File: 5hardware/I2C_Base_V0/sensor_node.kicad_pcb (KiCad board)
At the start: 2 copper layers, 99.5 x 99.5 mm, 264 parts, among them J2 PJ-320D-A, J3 Conn_02x06_Top_Bottom, J4 Conn_01x19_Socket, J5 Conn_01x19_Socket, J6 Conn_01x06_Socket, J7 Conn_01x04_Pin, J8 Conn_01x04_Pin, P1 S3B-PH-SM4-TB, P2 S4B-PH-SM4-TB, P3 S3B-PH-SM4-TB, Q2 Si2371EDS, Q3 Si2371EDS, SW2 SW_Push, SW3 SW_Push, U10 ESP-12F, U12 APDS-9960, U14 DS3231M, U3 CR2450, U4 CH32V003F4P6, U5 SHT31-DIS, U6 DS1307Z+, U7 XC6206PxxxMR, U8 TPL5110, U9 BH1750FVI-TR, Y1 Crystal, Y2 Crystal

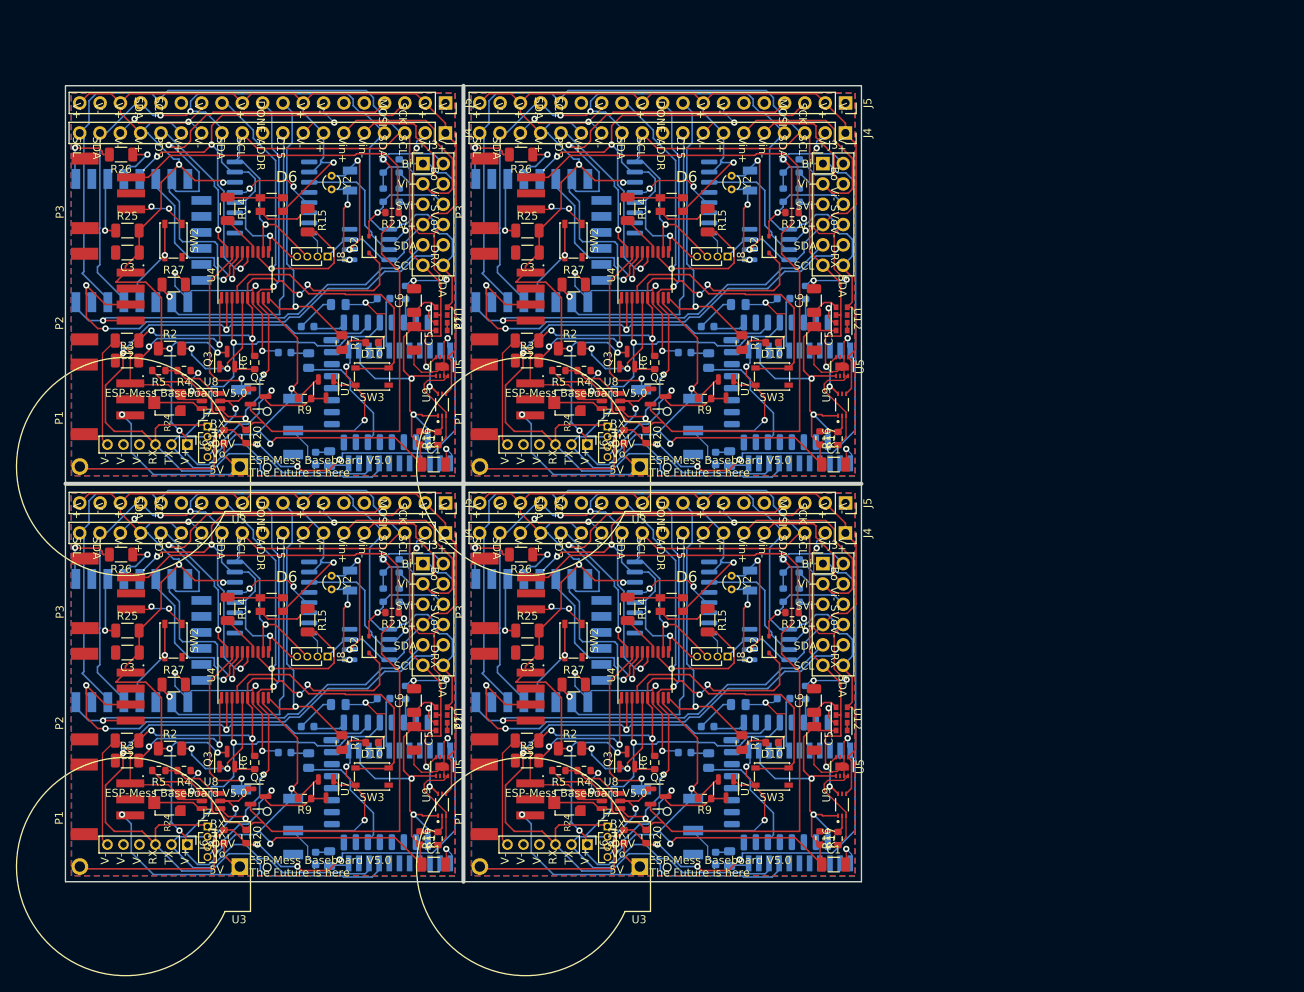
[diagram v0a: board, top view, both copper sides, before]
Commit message: update PCB.
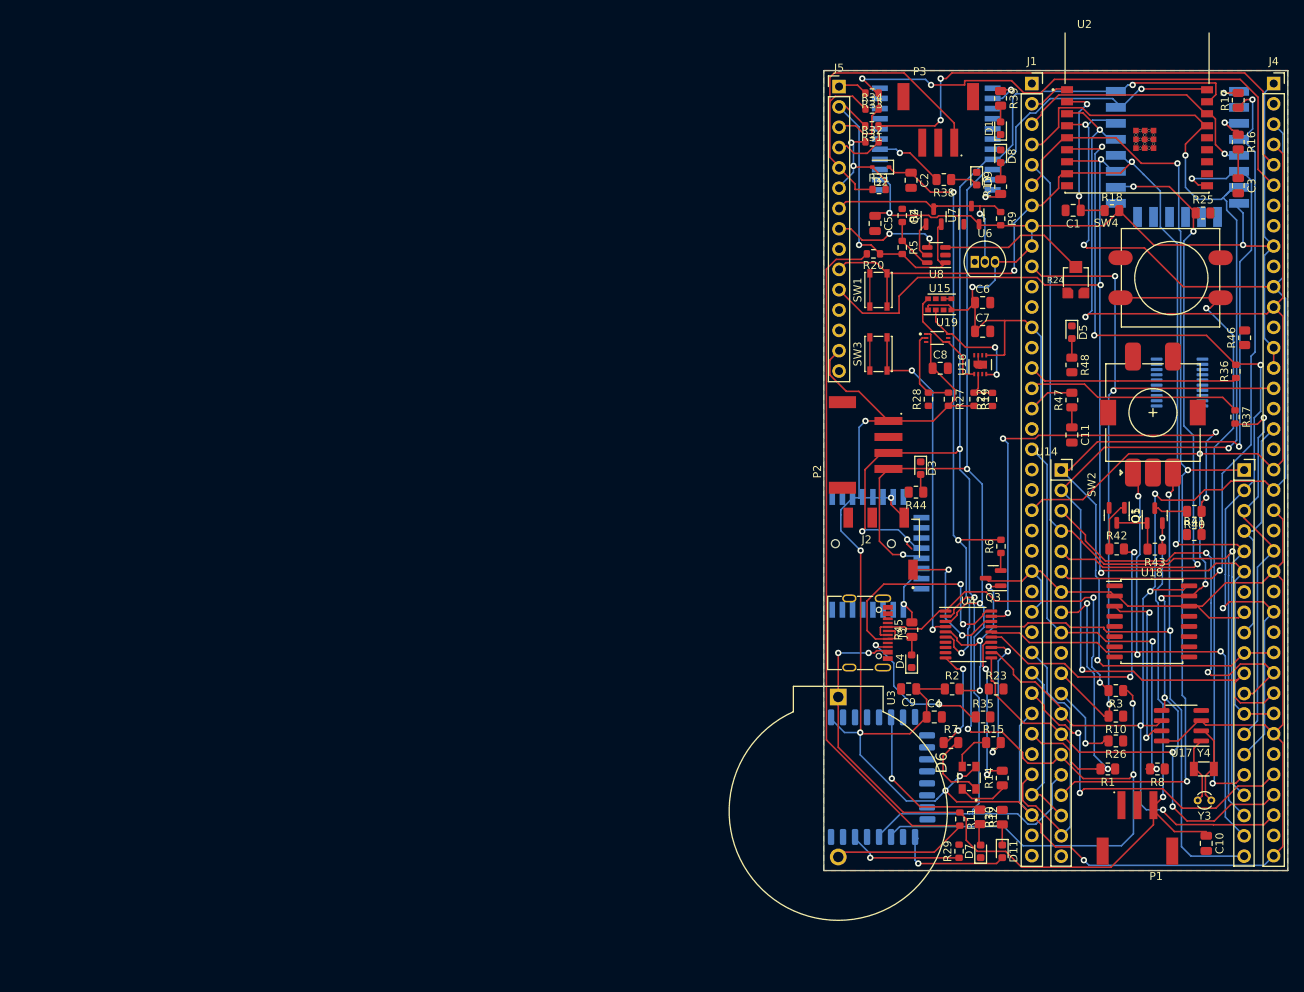
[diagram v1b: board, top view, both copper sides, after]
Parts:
- removed the C1 at (146.2, 141.2)
- removed the C1 at (96.2, 141.2)
- removed the C1 at (96.2, 91.2)
- removed the C1 at (146.2, 91.2)
- removed the C2 at (107.9, 75.8)
- removed the C2 at (57.9, 75.8)
- removed the C2 at (57.9, 125.8)
- removed the C2 at (107.9, 125.8)
- removed the C3 at (108.0, 64.8)
- removed the C3 at (58.0, 64.8)
- removed the C3 at (58.0, 114.8)
- removed the C3 at (108.0, 114.8)
- removed the C5 at (143.8, 125.5)
- removed the C5 at (93.8, 75.5)
- removed the C5 at (93.8, 125.5)
- removed the C5 at (143.8, 75.5)
- removed the C6 at (143.8, 70.8)
- removed the C6 at (93.8, 120.8)
- removed the C6 at (93.8, 70.8)
- removed the C6 at (143.8, 120.8)
- removed the D1 at (127.6, 77.2)
- removed the D1 at (127.6, 127.2)
- removed the D1 at (77.6, 77.2)
- removed the D1 at (77.6, 127.2)
- removed D10 (x4): LED, LED_SMD:LED_0603_1608Metric
- removed the D2 at (88.1, 113.8)
- removed the D2 at (138.1, 63.8)
- removed the D2 at (88.1, 63.8)
- removed the D2 at (138.1, 113.8)
- removed the D3 at (130.5, 124.0)
- removed the D3 at (80.5, 124.0)
- removed the D3 at (80.5, 74.0)
- removed the D3 at (130.5, 74.0)
- removed the D4 at (140.0, 120.5)
- removed the D4 at (90.0, 120.5)
- removed the D4 at (90.0, 70.5)
- removed the D4 at (140.0, 70.5)
- removed the D5 at (81.5, 90.5)
- removed the D5 at (131.5, 90.5)
- removed the D5 at (131.5, 140.5)
- removed the D5 at (81.5, 140.5)
- removed the D6 at (76.0, 108.8)
- removed the D6 at (126.0, 108.8)
- removed the D6 at (126.0, 58.8)
- removed the D6 at (76.0, 58.8)
- removed the J2 at (75.4, 87.7)
- removed the J2 at (125.4, 137.7)
- removed the J2 at (75.4, 137.7)
- removed the J2 at (125.4, 87.7)
- removed the J3 at (94.9, 53.6)
- removed the J3 at (144.9, 53.6)
- removed the J3 at (94.9, 103.6)
- removed the J3 at (144.9, 103.6)
- removed the J4 at (97.7, 99.8)
- removed the J4 at (97.7, 49.8)
- removed the J4 at (147.7, 99.8)
- removed the J4 at (147.7, 49.8)
- removed the J5 at (97.7, 46.0)
- removed the J5 at (147.7, 46.0)
- removed the J5 at (147.7, 96.0)
- removed the J5 at (97.7, 96.0)
- removed J6 (x4): Conn_01x06_Socket, Connector_PinHeader_2.00mm:PinHeader_1x06_P2.00mm_Vertical
- removed J7 (x4), J8 (x4): Conn_01x04_Pin, Connector_PinHeader_1.27mm:PinHeader_1x04_P1.27mm_Vertical
- removed the P1 at (58.3, 133.1)
- removed the P1 at (108.3, 83.1)
- removed the P1 at (108.3, 133.1)
- removed the P1 at (58.3, 83.1)
- removed the P2 at (58.4, 70.2)
- removed the P2 at (108.3, 70.2)
- removed the P2 at (108.3, 120.2)
- removed the P2 at (58.4, 120.2)
- removed the P3 at (108.4, 57.4)
- removed the P3 at (108.4, 107.3)
- removed the P3 at (58.4, 57.4)
- removed the P3 at (58.4, 107.3)
- removed the Q2 at (124.3, 82.8)
- removed the Q2 at (74.3, 132.8)
- removed the Q2 at (124.3, 132.8)
- removed the Q2 at (74.3, 82.8)
- removed the Q3 at (120.4, 78.1)
- removed the Q3 at (70.4, 128.1)
- removed the Q3 at (70.4, 78.1)
- removed the Q3 at (120.4, 128.1)
- removed the R1 at (142.7, 119.8)
- removed the R1 at (92.7, 119.8)
- removed the R1 at (92.7, 69.8)
- removed the R1 at (142.7, 69.8)
- removed the R10 at (133.2, 90.5)
- removed the R10 at (133.2, 140.5)
- removed the R10 at (83.2, 90.5)
- removed the R10 at (83.2, 140.5)
- removed the R11 at (70.0, 87.8)
- removed the R11 at (120.0, 137.8)
- removed the R11 at (120.0, 87.8)
- removed the R11 at (70.0, 137.8)
- removed the R14 at (120.5, 59.3)
- removed the R14 at (70.5, 59.3)
- removed the R14 at (70.5, 109.3)
- removed the R14 at (120.5, 109.3)
- removed the R15 at (130.5, 60.7)
- removed the R15 at (80.5, 60.7)
- removed the R15 at (80.5, 110.7)
- removed the R15 at (130.5, 110.7)
- removed the R16 at (96.8, 138.0)
- removed the R16 at (146.8, 88.0)
- removed the R16 at (96.8, 88.0)
- removed the R16 at (146.8, 138.0)
- removed the R17 at (144.5, 137.9)
- removed the R17 at (94.5, 87.9)
- removed the R17 at (144.5, 87.9)
- removed the R17 at (94.5, 137.9)
- removed the R18 at (91.9, 103.9)
- removed the R18 at (141.9, 53.9)
- removed the R18 at (91.9, 53.9)
- removed the R18 at (141.9, 103.9)
- removed the R19 at (139.9, 103.9)
- removed the R19 at (89.9, 53.9)
- removed the R19 at (139.9, 53.9)
- removed the R19 at (89.9, 103.9)
- removed the R2 at (113.3, 126.8)
- removed the R2 at (113.3, 76.8)
- removed the R2 at (63.3, 76.8)
- removed the R2 at (63.3, 126.8)
- removed the R20 at (72.8, 87.8)
- removed the R20 at (72.8, 137.8)
- removed the R20 at (122.8, 87.8)
- removed the R20 at (122.8, 137.8)
- removed the R21 at (141.0, 109.8)
- removed the R21 at (141.0, 59.8)
- removed the R21 at (91.0, 59.8)
- removed the R21 at (91.0, 109.8)
- removed the R22 at (91.9, 107.6)
- removed the R22 at (141.9, 107.6)
- removed the R22 at (141.9, 57.6)
- removed the R22 at (91.9, 57.6)
- removed the R23 at (89.9, 107.6)
- removed the R23 at (139.9, 107.6)
- removed the R23 at (89.9, 57.6)
- removed the R23 at (139.9, 57.6)
- removed the R24 at (113.0, 133.5)
- removed the R24 at (63.0, 133.5)
- removed the R24 at (113.0, 83.5)
- removed the R24 at (63.0, 83.5)
- removed the R25 at (108.0, 112.0)
- removed the R25 at (58.0, 62.0)
- removed the R25 at (58.0, 112.0)
- removed the R25 at (108.0, 62.0)
- removed the R26 at (57.1, 52.5)
- removed the R26 at (57.1, 102.5)
- removed the R26 at (107.1, 52.5)
- removed the R26 at (107.1, 102.5)
- removed the R27 at (113.7, 68.8)
- removed the R27 at (63.7, 118.8)
- removed the R27 at (63.7, 68.8)
- removed the R27 at (113.7, 118.8)
- removed the R28 at (134.3, 71.2)
- removed the R28 at (134.3, 121.2)
- removed the R28 at (84.3, 71.2)
- removed the R28 at (84.3, 121.2)
- removed the R3 at (57.9, 128.2)
- removed the R3 at (107.9, 128.2)
- removed the R3 at (57.9, 78.2)
- removed the R3 at (107.9, 78.2)
- removed the R4 at (65.0, 79.5)
- removed the R4 at (115.0, 129.5)
- removed the R4 at (65.0, 129.5)
- removed the R4 at (115.0, 79.5)
- removed the R5 at (61.9, 79.5)
- removed the R5 at (111.9, 79.5)
- removed the R5 at (111.9, 129.5)
- removed the R5 at (61.9, 129.5)
- removed the R6 at (123.9, 128.5)
- removed the R6 at (123.9, 78.5)
- removed the R6 at (73.9, 128.5)
- removed the R6 at (73.9, 78.5)
- removed the R7 at (84.8, 126.0)
- removed the R7 at (134.8, 76.0)
- removed the R7 at (84.8, 76.0)
- removed the R7 at (134.8, 126.0)
- removed the R8 at (130.6, 128.2)
- removed the R8 at (80.6, 128.2)
- removed the R8 at (130.6, 78.2)
- removed the R8 at (80.6, 78.2)
- removed the R9 at (80.1, 133.0)
- removed the R9 at (130.1, 133.0)
- removed the R9 at (80.1, 83.0)
- removed the R9 at (130.1, 83.0)
- removed the SW2 at (63.7, 63.2)
- removed the SW2 at (113.7, 113.2)
- removed the SW2 at (113.7, 63.2)
- removed the SW2 at (63.7, 113.2)
- removed the SW3 at (88.5, 80.2)
- removed the SW3 at (88.5, 130.2)
- removed the SW3 at (138.5, 130.2)
- removed the SW3 at (138.5, 80.2)
- removed the U10 at (48.9, 105.2)
- removed the U10 at (48.9, 55.2)
- removed the U10 at (98.9, 55.2)
- removed the U10 at (98.9, 105.2)
- removed the U11 at (83.5, 73.5)
- removed the U11 at (83.5, 123.5)
- removed the U11 at (133.5, 73.5)
- removed the U11 at (133.5, 123.5)
- removed U12 (x4): APDS-9960, Sensor:Avago_APDS-9960
- removed the U14 at (76.0, 107.9)
- removed the U14 at (126.0, 107.9)
- removed the U14 at (76.0, 57.9)
- removed the U14 at (126.0, 57.9)
- removed the U2 at (99.2, 92.3)
- removed the U2 at (99.2, 142.3)
- removed the U2 at (149.2, 92.3)
- removed the U2 at (149.2, 142.3)
- removed the U3 at (122.0, 141.5)
- removed the U3 at (72.0, 91.5)
- removed the U3 at (122.0, 91.5)
- removed the U3 at (72.0, 141.5)
- removed the U4 at (72.6, 67.5)
- removed the U4 at (122.6, 67.5)
- removed the U4 at (72.6, 117.5)
- removed the U4 at (122.6, 117.5)
- removed the U5 at (97.3, 79.0)
- removed the U5 at (147.3, 79.0)
- removed the U5 at (97.3, 129.0)
- removed the U5 at (147.3, 129.0)
- removed the U6 at (138.2, 63.8)
- removed the U6 at (88.2, 63.8)
- removed the U6 at (88.2, 113.8)
- removed the U6 at (138.2, 113.8)
- removed the U7 at (132.8, 81.8)
- removed the U7 at (82.8, 81.8)
- removed the U7 at (82.8, 131.8)
- removed the U7 at (132.8, 131.8)
- removed the U8 at (68.4, 133.3)
- removed the U8 at (118.4, 83.3)
- removed the U8 at (68.4, 83.3)
- removed the U8 at (118.4, 133.3)
- removed the U9 at (147.3, 133.8)
- removed the U9 at (147.3, 83.8)
- removed the U9 at (97.3, 133.8)
- removed the U9 at (97.3, 83.8)
- removed Y1 (x4): Crystal, Crystal:Crystal_SMD_3215-2Pin_3.2x1.5mm
- removed Y2 (x4): Crystal, Crystal:Crystal_Round_D1.5mm_Vertical
- added C1: C, Capacitor_SMD:C_0805_2012Metric, F.Cu at (176.2, 59.5)
- added C10: C, Capacitor_SMD:C_0805_2012Metric, F.Cu at (192.8, 138.6)
- added C11: C, Capacitor_SMD:C_0805_2012Metric, F.Cu at (176.0, 87.5)
- added C2: C, Capacitor_SMD:C_0805_2012Metric, F.Cu at (155.9, 55.7)
- added C3: C, Capacitor_SMD:C_0805_2012Metric, F.Cu at (196.8, 56.4)
- added C4: C, Capacitor_SMD:C_0805_2012Metric, F.Cu at (158.8, 122.8)
- added C5: C, Capacitor_SMD:C_0805_2012Metric, F.Cu at (151.4, 61.1)
- added C6: C, Capacitor_SMD:C_0805_2012Metric, F.Cu at (164.8, 71.0)
- added C7: C, Capacitor_SMD:C_0805_2012Metric, F.Cu at (164.8, 74.6)
- added C8: C, Capacitor_SMD:C_0805_2012Metric, F.Cu at (159.5, 79.2)
- added C9: C, Capacitor_SMD:C_0805_2012Metric, F.Cu at (155.6, 119.3)
- added D1: LED, LED_SMD:LED_0603_1608Metric, F.Cu at (167.1, 49.2)
- added D11: LED, LED_SMD:LED_0603_1608Metric, F.Cu at (167.3, 139.6)
- added D2: D_Schottky, Diode_SMD:D_SOD-323, F.Cu at (152.1, 54.1)
- added D3: LED, LED_SMD:LED_0603_1608Metric, F.Cu at (157.1, 91.7)
- added D4: LED, LED_SMD:LED_0603_1608Metric, F.Cu at (156.0, 115.8)
- added D5: LED, LED_SMD:LED_0603_1608Metric, F.Cu at (176.0, 74.7)
- added D6: LL-R3528RGBC-008-B, R3528RGB:LED_LL-R3528RGBC-008-B, F.Cu at (163.2, 130.4)
- added D7: LED, LED_SMD:LED_0603_1608Metric, F.Cu at (164.6, 139.6)
- added D8: LED, LED_SMD:LED_0603_1608Metric, F.Cu at (167.1, 52.7)
- added D9: LED, LED_SMD:LED_0603_1608Metric, F.Cu at (164.1, 55.5)
- added J1: Conn_01x39_Socket, Connector_PinSocket_2.54mm:PinSocket_1x39_P2.54mm_Vertical, F.Cu at (171.0, 43.6)
- added J2: PJ-320D-A, A_SensorNode:PJ-320D, F.Cu at (150.3, 101.1)
- added J3: USB_C_Receptacle_USB2.0, Connector_USB:USB_C_Receptacle_G-Switch_GT-USB-7010ASV, F.Cu at (149.3, 112.3)
- added J4: Conn_01x39_Socket, Connector_PinSocket_2.54mm:PinSocket_1x39_P2.54mm_Vertical, F.Cu at (201.2, 43.6)
- added J5: Conn_01x15_Pin, Connector_PinHeader_2.54mm:PinHeader_1x15_P2.54mm_Vertical, F.Cu at (146.9, 44.0)
- added P1: S3B-PH-SM4-TB, S3B-PH:JST_S3B-PH-SM4-TB, F.Cu at (184.2, 133.8)
- added P2: S4B-PH-SM4-TB, S4B-PH:JST_S4B-PH-SM4-TB, F.Cu at (153.1, 88.8)
- added P3: S3B-PH-SM4-TB, S3B-PH:JST_S3B-PH-SM4-TB, F.Cu at (159.3, 51.0)
- added Q1: Si2371EDS, Package_TO_SOT_SMD:SOT-23, F.Cu at (186.4, 97.6)
- added Q2: Si2371EDS, Package_TO_SOT_SMD:SOT-23, F.Cu at (158.7, 60.3)
- added Q3: Si2371EDS, Package_TO_SOT_SMD:SOT-23, F.Cu at (166.2, 105.5)
- added Q5: MMBT5551L, Package_TO_SOT_SMD:SOT-23, F.Cu at (181.6, 97.6)
- added R1: R, Resistor_SMD:R_0805_2012Metric, F.Cu at (180.5, 129.3)
- added R10: R, Resistor_SMD:R_0805_2012Metric, F.Cu at (181.5, 122.7)
- added R11: R, Resistor_SMD:R_0603_1608Metric, F.Cu at (162.0, 135.6)
- added R12: R, Resistor_SMD:R_0805_2012Metric, F.Cu at (164.5, 135.3)
- added R13: R, Resistor_SMD:R_0805_2012Metric, F.Cu at (167.1, 56.5)
- added R14: R, Resistor_SMD:R_0805_2012Metric, F.Cu at (167.3, 130.4)
- added R15: R, Resistor_SMD:R_0805_2012Metric, F.Cu at (166.2, 126.0)
- added R16: R, Resistor_SMD:R_0805_2012Metric, F.Cu at (196.8, 50.9)
- added R17: R, Resistor_SMD:R_0805_2012Metric, F.Cu at (196.8, 45.7)
- added R18: R, Resistor_SMD:R_0805_2012Metric, F.Cu at (181.0, 59.5)
- added R19: R, Resistor_SMD:R_0603_1608Metric, F.Cu at (163.8, 83.1)
- added R2: R, Resistor_SMD:R_0805_2012Metric, F.Cu at (161.0, 119.3)
- added R20: R, Resistor_SMD:R_0603_1608Metric, F.Cu at (151.2, 64.9)
- added R21: R, Resistor_SMD:R_0603_1608Metric, F.Cu at (151.9, 56.9)
- added R22: R, Resistor_SMD:R_0603_1608Metric, F.Cu at (166.1, 83.1)
- added R23: R, Resistor_SMD:R_0805_2012Metric, F.Cu at (166.5, 119.3)
- added R24: EVM3ESX50B12, EVM3ES:EMV3ESX50B12, F.Cu at (176.5, 68.2)
- added R25: R, Resistor_SMD:R_0805_2012Metric, F.Cu at (192.4, 59.8)
- added R26: R, Resistor_SMD:R_0805_2012Metric, F.Cu at (181.5, 125.8)
- added R27: R, Resistor_SMD:R_0603_1608Metric, F.Cu at (160.6, 83.1)
- added R28: R, Resistor_SMD:R_0603_1608Metric, F.Cu at (158.1, 83.1)
- added R29: R, Resistor_SMD:R_0603_1608Metric, F.Cu at (161.9, 139.6)
- added R3: R, Resistor_SMD:R_0805_2012Metric, F.Cu at (181.5, 119.5)
- added R30: R, Resistor_SMD:R_0805_2012Metric, F.Cu at (167.3, 135.3)
- added R31: R, Resistor_SMD:R_0603_1608Metric, F.Cu at (151.0, 48.9)
- added R32: R, Resistor_SMD:R_0603_1608Metric, F.Cu at (151.0, 50.9)
- added R33: R, Resistor_SMD:R_0603_1608Metric, F.Cu at (151.0, 44.8)
- added R34: R, Resistor_SMD:R_0603_1608Metric, F.Cu at (151.0, 46.8)
- added R35: R, Resistor_SMD:R_0805_2012Metric, F.Cu at (164.9, 122.8)
- added R36: R, Resistor_SMD:R_0603_1608Metric, F.Cu at (196.5, 79.6)
- added R37: R, Resistor_SMD:R_0603_1608Metric, F.Cu at (196.4, 85.3)
- added R38: R, Resistor_SMD:R_0805_2012Metric, F.Cu at (160.0, 55.6)
- added R39: R, Resistor_SMD:R_0805_2012Metric, F.Cu at (167.1, 45.5)
- added R4: R, Resistor_SMD:R_0603_1608Metric, F.Cu at (154.8, 60.1)
- added R40: R, Resistor_SMD:R_0805_2012Metric, F.Cu at (191.3, 97.1)
- added R41: R, Resistor_SMD:R_0805_2012Metric, F.Cu at (191.3, 100.0)
- added R42: R, Resistor_SMD:R_0805_2012Metric, F.Cu at (181.6, 101.8)
- added R43: R, Resistor_SMD:R_0805_2012Metric, F.Cu at (186.4, 101.8)
- added R44: R, Resistor_SMD:R_0805_2012Metric, F.Cu at (156.5, 94.7)
- added R45: R, Resistor_SMD:R_0805_2012Metric, F.Cu at (156.0, 111.9)
- added R46: R, Resistor_SMD:R_0805_2012Metric, F.Cu at (197.6, 75.4)
- added R47: R, Resistor_SMD:R_0805_2012Metric, F.Cu at (176.0, 83.2)
- added R48: R, Resistor_SMD:R_0805_2012Metric, F.Cu at (176.0, 78.8)
- added R5: R, Resistor_SMD:R_0603_1608Metric, F.Cu at (154.8, 64.1)
- added R6: R, Resistor_SMD:R_0603_1608Metric, F.Cu at (167.1, 101.5)
- added R7: R, Resistor_SMD:R_0805_2012Metric, F.Cu at (160.9, 126.0)
- added R8: R, Resistor_SMD:R_0805_2012Metric, F.Cu at (186.7, 129.3)
- added R9: R, Resistor_SMD:R_0603_1608Metric, F.Cu at (167.1, 60.5)
- added SW1: SW_Push, Button_Switch_SMD:SW_SPST_PTS810, F.Cu at (151.8, 69.4)
- added SW2: RotaryEncoder, A_SensorNode:RotaryEncoder_E11, F.Cu at (179.0, 93.8)
- added SW3: SW_Push, Button_Switch_SMD:SW_SPST_PTS810, F.Cu at (151.8, 77.4)
- added SW4: SW_Push, A_SensorNode:ButtonSwitch12mm_SMD, F.Cu at (180.3, 61.5)
- added U1: ~, A_SensorNode:JDY-Base, B.Cu at (157.9, 137.8)
- added U10: ESP-12F, A_SensorNode:ESP12_SMD, B.Cu at (197.2, 42.0)
- added U11: STM32L010F4Px, Package_SO:TSSOP-20_4.4x6.5mm_P0.65mm, B.Cu at (189.5, 81.0)
- added U14: Lolin_Base, A_SensorNode:LolinBase, F.Cu at (172.9, 90.1)
- added U15: APDS-9960, Sensor:Avago_APDS-9960, F.Cu at (159.5, 71.2)
- added U16: SHT31-DIS, Sensor_Humidity:Sensirion_DFN-8-1EP_2.5x2.5mm_P0.5mm_EP1.1x1.7mm, F.Cu at (164.5, 78.8)
- added U17: DS1307Z+, Package_SO:SOIC-8_3.9x4.9mm_P1.27mm, F.Cu at (189.7, 123.9)
- added U18: DS3231M, Package_SO:SOIC-16W_7.5x10.3mm_P1.27mm, F.Cu at (186.0, 110.9)
- added U19: BH1750FVI-TR, BH1750:XDCR_BH1750FVI-TR, F.Cu at (159.2, 75.4)
- added U2: ESP32-C3-WROOM-02, ESP32-C3:MODULE_ESP32-C3-WROOM-02-H4, F.Cu at (184.2, 47.3)
- added U3: CR2450, Battery:BatteryHolder_ComfortableElectronic_CH273-2450_1x2450, F.Cu at (146.8, 120.3)
- added U4: CH32V003F4P6, Package_SO:TSSOP-20_4.4x6.5mm_P0.65mm, F.Cu at (163.1, 112.5)
- added U5: ~, A_SensorNode:E104-BT07, B.Cu at (167.3, 43.3)
- added U6: MCP1700x-330xxTO, Package_TO_SOT_THT:TO-92_Inline, F.Cu at (163.9, 65.9)
- added U7: XC6206PxxxMR, Package_TO_SOT_SMD:SOT-23-3, F.Cu at (163.4, 60.1)
- added U8: TPL5110, Package_TO_SOT_SMD:SOT-23-6, F.Cu at (159.1, 65.1)
- added U9: E18-MS1-PCB, RF_Module:E18-MS1-PCB, B.Cu at (145.7, 102.3)
- added Y3: Crystal, Crystal:Crystal_Round_D1.5mm_Vertical, F.Cu at (193.4, 133.2)
- added Y4: Crystal, Crystal:Crystal_SMD_3215-2Pin_3.2x1.5mm, F.Cu at (192.5, 129.3)
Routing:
- net GND: track 846.6 -> 10.2 mm, vias 84 -> 0
- net VCC: track 1176.6 -> 473.6 mm, vias 40 -> 10
- net SCL (5): track 639.4 -> 0.00 mm, vias 16 -> 0
- net SDA (4): track 571.9 -> 0.00 mm, vias 12 -> 0
- net RX: track 393.2 -> 0.00 mm, vias 8 -> 0
- net TX: track 303.7 -> 0.00 mm, vias 4 -> 0
- net Bat-Vo: track 330.9 -> 40.6 mm, vias 4 -> 1
- net Bat-Vi: track 380.1 -> 106.5 mm, vias 12 -> 0
- net D3_RX: track 243.9 -> 0.00 mm, vias 8 -> 0
- net SDA0: track 0.00 -> 243.6 mm, vias 0 -> 8
- net RX1: track 0.00 -> 223.5 mm, vias 0 -> 8
- net SCL0: track 0.00 -> 217.3 mm, vias 0 -> 8
- net D1_TX: track 209.1 -> 0.00 mm, vias 4 -> 0
- net TX1: track 0.00 -> 177.9 mm, vias 0 -> 4
- net DONE: track 190.1 -> 13.7 mm, vias 12 -> 2
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- removed copper zone on B.Cu, net GND
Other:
- board size 99.5 x 99.5 mm -> 58 x 100 mm
- board text removed: "5V"
- board text removed: "ADDR"
- board text removed: "Bi"
- board text removed: "Bo"
- board text removed: "D15"
- board text removed: "DONE"
- board text removed: "DRV"
- board text removed: "DRX"
- board text removed: "DTX"
- board text removed: "ESP-Mess Baseboard V5.0"
- board text removed: "MOSI"
- board text removed: "PD2"
- board text removed: "RX"
- board text removed: "SCK"
- board text removed: "SCL"
- board text removed: "SDA"
- board text removed: "SVi"
- board text removed: "SVo"
- board text removed: "TX"
- board text removed: "The Future is here"
- board text removed: "V+"
- board text removed: "V-"
- board text removed: "V-CUT"
- board text removed: "Vi+"
- board text removed: "Vi-"
- board text removed: "Vin+"
- board text removed: "Vin-"
- board text removed: "Vo"
